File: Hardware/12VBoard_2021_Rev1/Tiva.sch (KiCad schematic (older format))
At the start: 2 parts

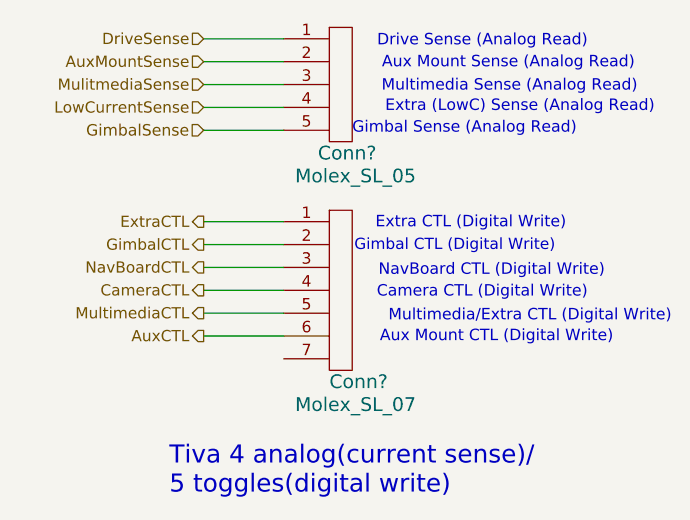
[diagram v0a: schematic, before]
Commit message: fixed some stuffs
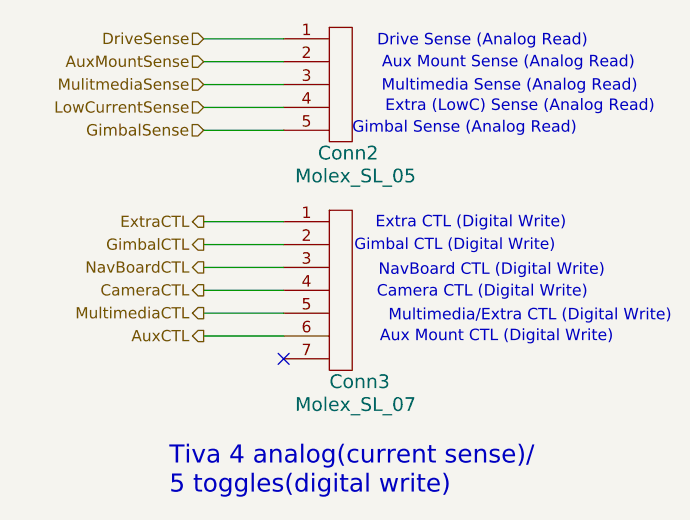
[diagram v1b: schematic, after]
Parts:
- Conn2: renamed from Conn?; footprint (none) -> MRDT_Connectors:MOLEX_SL_05_Horizontal
- Conn3: renamed from Conn?; footprint (none) -> MRDT_Connectors:MOLEX_SL_07_Horizontal
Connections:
- no-connect marks 0 -> 1
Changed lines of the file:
@@
 	6150 2250 5800 2250
 $Comp
-L MRDT_Connectors:Molex_SL_05 Conn?
+L MRDT_Connectors:Molex_SL_05 Conn2
 U 1 1 5F976F73
 P 6350 1900
-F 0 "Conn?" H 6300 1850 60  0000 L CNN
+F 0 "Conn2" H 6300 1850 60  0000 L CNN
 F 1 "Molex_SL_05" H 6200 1750 60  0000 L CNN
-F 2 "" H 6350 1900 60  0001 C CNN
+F 2 "MRDT_Connectors:MOLEX_SL_05_Horizontal" H 6350 1900 60  0001 C CNN
 F 3 "" H 6350 1900 60  0001 C CNN
 	1    6350 1900
@@
 $EndComp
 $Comp
-L MRDT_Connectors:Molex_SL_07 Conn?
+L MRDT_Connectors:Molex_SL_07 Conn3
 U 1 1 5F97771C
 P 6350 2900
-F 0 "Conn?" H 6350 2850 60  0000 L CNN
+F 0 "Conn3" H 6350 2850 60  0000 L CNN
 F 1 "Molex_SL_07" H 6200 2750 60  0000 L CNN
-F 2 "" H 6350 3100 60  0001 C CNN
+F 2 "MRDT_Connectors:MOLEX_SL_07_Horizontal" H 6350 3100 60  0001 C CNN
 F 3 "" H 6350 3100 60  0001 C CNN
 	1    6350 2900
@@
 Text Notes 6450 1872 0    50   ~ 0
 Gimbal Sense (Analog Read)
+NoConn ~ 6150 2850
 $EndSCHEMATC
